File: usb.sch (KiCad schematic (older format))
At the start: 0 parts

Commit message: add control
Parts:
- added U?: MCIMX6Y2DVM, symbol MCIMX6Y2DVM
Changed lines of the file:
@@
 $Descr A4 11693 8268
 encoding utf-8
-Sheet 1 10
+Sheet 5 11
 Title ""
 Date ""
@@
 Comment4 ""
 $EndDescr
+$Comp
+L MCIMX6Y2DVM U?
+U 11 1 5A0FE973
+P 5200 3100
+F 0 "U?" H 5200 3387 60  0000 C CNN
+F 1 "MCIMX6Y2DVM" H 5200 3281 60  0000 C CNN
+F 2 "" H 3050 2100 60  0001 C CNN
+F 3 "" H 3050 2100 60  0001 C CNN
+	11   5200 3100
+	1    0    0    -1
+$EndComp
 $EndSCHEMATC

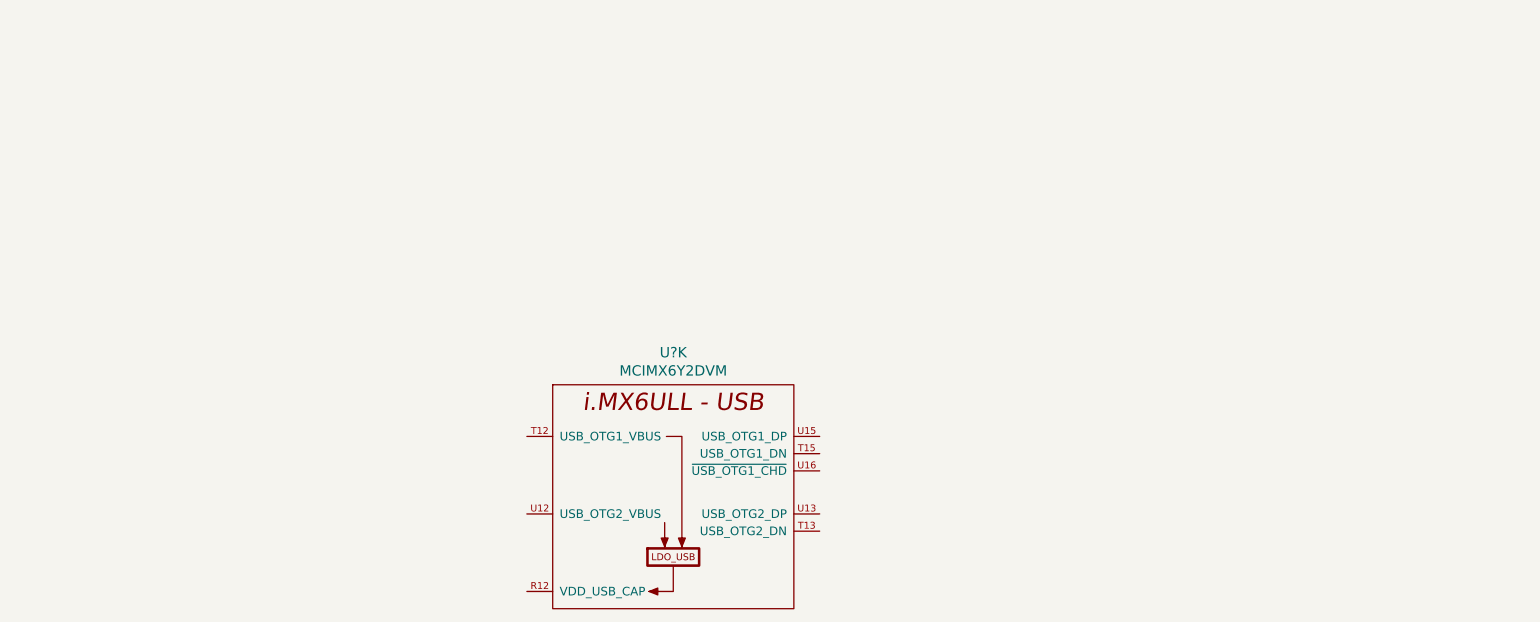
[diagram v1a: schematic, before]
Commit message: start some usb
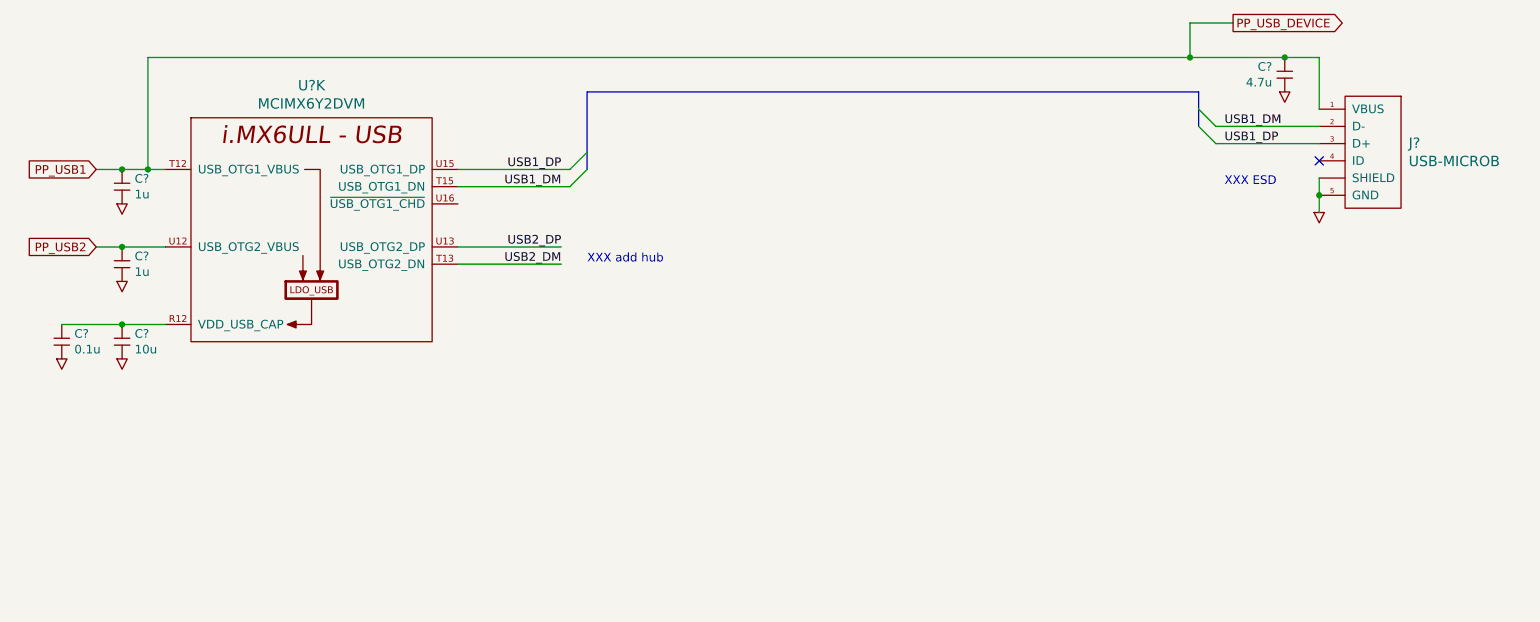
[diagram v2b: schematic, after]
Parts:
- added C?: 0.1u, symbol C
- added C?: 10u, symbol C
- added C? (x2): 1u, symbol C
- added C?: 4.7u, symbol C
- added J?: USB-MICROB, symbol USB-MICROB
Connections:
- net at U?.R12 (VDD_USB_CAP): now also C?.1, C?.1
- net PP_USB1: now reaches U?.T12 (USB_OTG1_VBUS)
- net PP_USB1: now also C?.1, C?.1, J?.1 (VBUS)
- net USB2_DM: now reaches U?.T13 (USB_OTG2_DN)
- net USB1_DM: now reaches U?.T15 (USB_OTG1_DN)
- net USB1_DM: now also J?.2 (D-)
- net PP_USB2: now reaches U?.U12 (USB_OTG2_VBUS)
- net PP_USB2: now also C?.1
- net USB2_DP: now reaches U?.U13 (USB_OTG2_DP)
- net USB1_DP: now reaches U?.U15 (USB_OTG1_DP)
- net USB1_DP: now also J?.3 (D+)
- new net COM: C?.2, C?.2, C?.2, C?.2, C?.2, J?.5 (GND), J?.SHIE (SHIELD)
- no-connect marks 0 -> 1
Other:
- note added: "XXX ESD"
- note added: "XXX add hub"
- moved on the sheet: U?K
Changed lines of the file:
@@
 L MCIMX6Y2DVM U?
 U 11 1 5A0FE973
-P 5200 3100
-F 0 "U?" H 5200 3387 60  0000 C CNN
-F 1 "MCIMX6Y2DVM" H 5200 3281 60  0000 C CNN
-F 2 "" H 3050 2100 60  0001 C CNN
-F 3 "" H 3050 2100 60  0001 C CNN
-	11   5200 3100
-	1    0    0    -1
-$EndComp
+P 3100 1550
+F 0 "U?" H 3100 1837 60  0000 C CNN
+F 1 "MCIMX6Y2DVM" H 3100 1731 60  0000 C CNN
+F 2 "" H 950 550 60  0001 C CNN
+F 3 "" H 950 550 60  0001 C CNN
+	11   3100 1550
+	1    0    0    -1
+$EndComp
+$Comp
+L C C?
+U 1 1 5A198FE1
+P 1650 2650
+F 0 "C?" H 1723 2596 50  0000 L CNN
+F 1 "0.1u" H 1723 2505 50  0000 L CNN
+F 2 "" H 1550 2800 60  0000 C CNN
+F 3 "" H 1550 2800 60  0000 C CNN
+	1    1650 2650
+	1    0    0    -1
+$EndComp
+$Comp
+L C C?
+U 1 1 5A19904E
+P 2000 2650
+F 0 "C?" H 2073 2596 50  0000 L CNN
+F 1 "10u" H 2073 2505 50  0000 L CNN
+F 2 "" H 1900 2800 60  0000 C CNN
+F 3 "" H 1900 2800 60  0000 C CNN
+	1    2000 2650
+	1    0    0    -1
+$EndComp
+$Comp
+L COM #PWR?
+U 1 1 5A19917F
+P 2000 2850
+F 0 "#PWR?" V 2275 2850 60  0001 C CNN
+F 1 "COM" H 2160 2735 30  0001 C CNN
+F 2 "" H 2155 2860 60  0000 C CNN
+F 3 "" H 2155 2860 60  0000 C CNN
+	1    2000 2850
+	1    0    0    -1
+$EndComp
+$Comp
+L COM #PWR?
+U 1 1 5A199197
+P 1650 2850
+F 0 "#PWR?" V 1925 2850 60  0001 C CNN
+F 1 "COM" H 1810 2735 30  0001 C CNN
+F 2 "" H 1805 2860 60  0000 C CNN
+F 3 "" H 1805 2860 60  0000 C CNN
+	1    1650 2850
+	1    0    0    -1
+$EndComp
+Wire Wire Line
+	1650 2650 2250 2650
+Connection ~ 2000 2650
+Text GLabel 1850 2200 0    50   Input ~ 0
+PP_USB2
+$Comp
+L C C?
+U 1 1 5A1994E4
+P 2000 2200
+F 0 "C?" H 2073 2146 50  0000 L CNN
+F 1 "1u" H 2073 2055 50  0000 L CNN
+F 2 "" H 1900 2350 60  0000 C CNN
+F 3 "" H 1900 2350 60  0000 C CNN
+	1    2000 2200
+	1    0    0    -1
+$EndComp
+Wire Wire Line
+	1850 2200 2250 2200
+Connection ~ 2000 2200
+$Comp
+L COM #PWR?
+U 1 1 5A199530
+P 2000 2400
+F 0 "#PWR?" V 2275 2400 60  0001 C CNN
+F 1 "COM" H 2160 2285 30  0001 C CNN
+F 2 "" H 2155 2410 60  0000 C CNN
+F 3 "" H 2155 2410 60  0000 C CNN
+	1    2000 2400
+	1    0    0    -1
+$EndComp
+Text GLabel 1850 1750 0    50   Input ~ 0
+PP_USB1
+$Comp
+L C C?
+U 1 1 5A1995A8
+P 2000 1750
+F 0 "C?" H 2073 1696 50  0000 L CNN
+F 1 "1u" H 2073 1605 50  0000 L CNN
+F 2 "" H 1900 1900 60  0000 C CNN
+F 3 "" H 1900 1900 60  0000 C CNN
+	1    2000 1750
+	1    0    0    -1
+$EndComp
+Wire Wire Line
+	1850 1750 2250 1750
+Connection ~ 2000 1750
+$Comp
+L COM #PWR?
+U 1 1 5A1995B1
+P 2000 1950
+F 0 "#PWR?" V 2275 1950 60  0001 C CNN
+F 1 "COM" H 2160 1835 30  0001 C CNN
+F 2 "" H 2155 1960 60  0000 C CNN
+F 3 "" H 2155 1960 60  0000 C CNN
+	1    2000 1950
+	1    0    0    -1
+$EndComp
+Wire Wire Line
+	3950 2200 4550 2200
+Wire Wire Line
+	4550 2300 3950 2300
+Text Label 4550 2200 2    50   ~ 0
+USB2_DP
+Text Label 4550 2300 2    50   ~ 0
+USB2_DM
+Text Notes 4700 2300 0    50   ~ 0
+XXX add hub
+$Comp
+L USB-MICROB J?
+U 1 1 5A1B6AF4
+P 9250 1650
+F 0 "J?" H 9031 1703 60  0000 R CNN
+F 1 "USB-MICROB" H 9031 1597 60  0000 R CNN
+F 2 "" H 9350 1300 60  0000 C CNN
+F 3 "" H 9350 1300 60  0000 C CNN
+	1    9250 1650
+	-1   0    0    -1
+$EndComp
+Text GLabel 8450 900  2    50   Output ~ 0
+PP_USB_DEVICE
+Wire Wire Line
+	2150 1100 8950 1100
+Wire Wire Line
+	8950 1100 8950 1400
+$Comp
+L C C?
+U 1 1 5A1B6D00
+P 8750 1100
+F 0 "C?" H 8823 1046 50  0000 L CNN
+F 1 "4.7u" H 8823 955 50  0000 L CNN
+F 2 "" H 8650 1250 60  0000 C CNN
+F 3 "" H 8650 1250 60  0000 C CNN
+	1    8750 1100
+	-1   0    0    -1
+$EndComp
+$Comp
+L COM #PWR?
+U 1 1 5A1B6EAA
+P 8750 1300
+F 0 "#PWR?" V 9025 1300 60  0001 C CNN
+F 1 "COM" H 8910 1185 30  0001 C CNN
+F 2 "" H 8905 1310 60  0000 C CNN
+F 3 "" H 8905 1310 60  0000 C CNN
+	1    8750 1300
+	1    0    0    -1
+$EndComp
+Text Notes 8400 1850 0    50   ~ 0
+XXX ESD
+Wire Wire Line
+	3950 1750 4600 1750
+Text Label 4550 1750 2    50   ~ 0
+USB1_DP
+Wire Wire Line
+	3950 1850 4600 1850
+Text Label 4550 1850 2    50   ~ 0
+USB1_DM
+Wire Wire Line
+	8950 1600 8350 1600
+Wire Wire Line
+	8950 1500 8350 1500
+NoConn ~ 8950 1700
+$Comp
+L COM #PWR?
+U 1 1 5A1B703E
+P 8950 2000
+F 0 "#PWR?" V 9225 2000 60  0001 C CNN
+F 1 "COM" H 9110 1885 30  0001 C CNN
+F 2 "" H 9105 2010 60  0000 C CNN
+F 3 "" H 9105 2010 60  0000 C CNN
+	1    8950 2000
+	1    0    0    -1
+$EndComp
+Wire Wire Line
+	8950 1900 8950 1900
+Wire Wire Line
+	8950 1800 8950 2000
+Connection ~ 8750 1100
+Connection ~ 8950 1900
+Entry Wire Line
+	4600 1750 4700 1650
+Entry Wire Line
+	4600 1850 4700 1750
+Entry Wire Line
+	8350 1500 8250 1400
+Entry Wire Line
+	8350 1600 8250 1500
+Text Label 8400 1600 0    50   ~ 0
+USB1_DP
+Wire Bus Line
+	4700 1300 4700 1750
+Wire Bus Line
+	8250 1300 8250 1500
+Wire Bus Line
+	8250 1300 4700 1300
+Wire Wire Line
+	8450 900  8200 900
+Wire Wire Line
+	8200 900  8200 1100
+Connection ~ 8200 1100
+Wire Wire Line
+	2150 1100 2150 1750
+Connection ~ 2150 1750
+Text Label 8400 1500 0    50   ~ 0
+USB1_DM
 $EndSCHEMATC
